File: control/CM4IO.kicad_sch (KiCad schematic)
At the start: 1 part

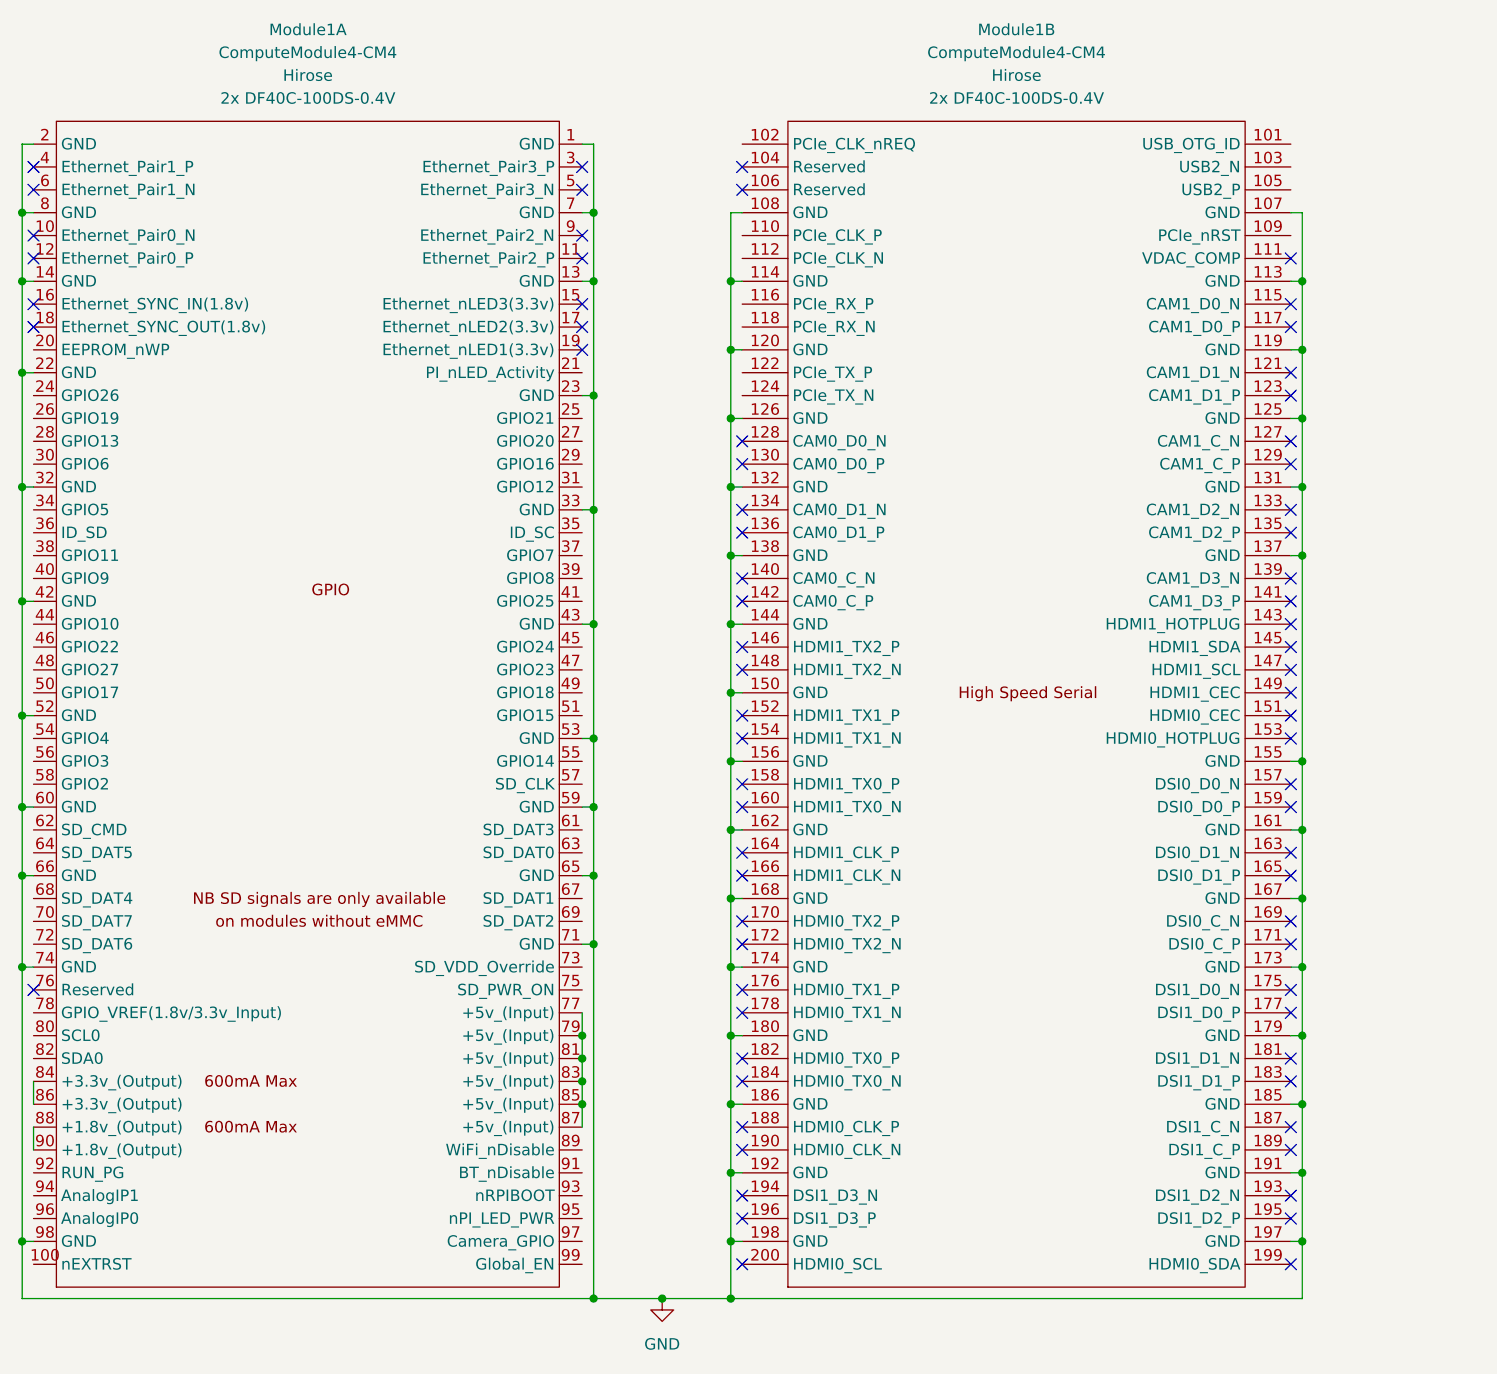
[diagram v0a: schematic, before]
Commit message: SSD
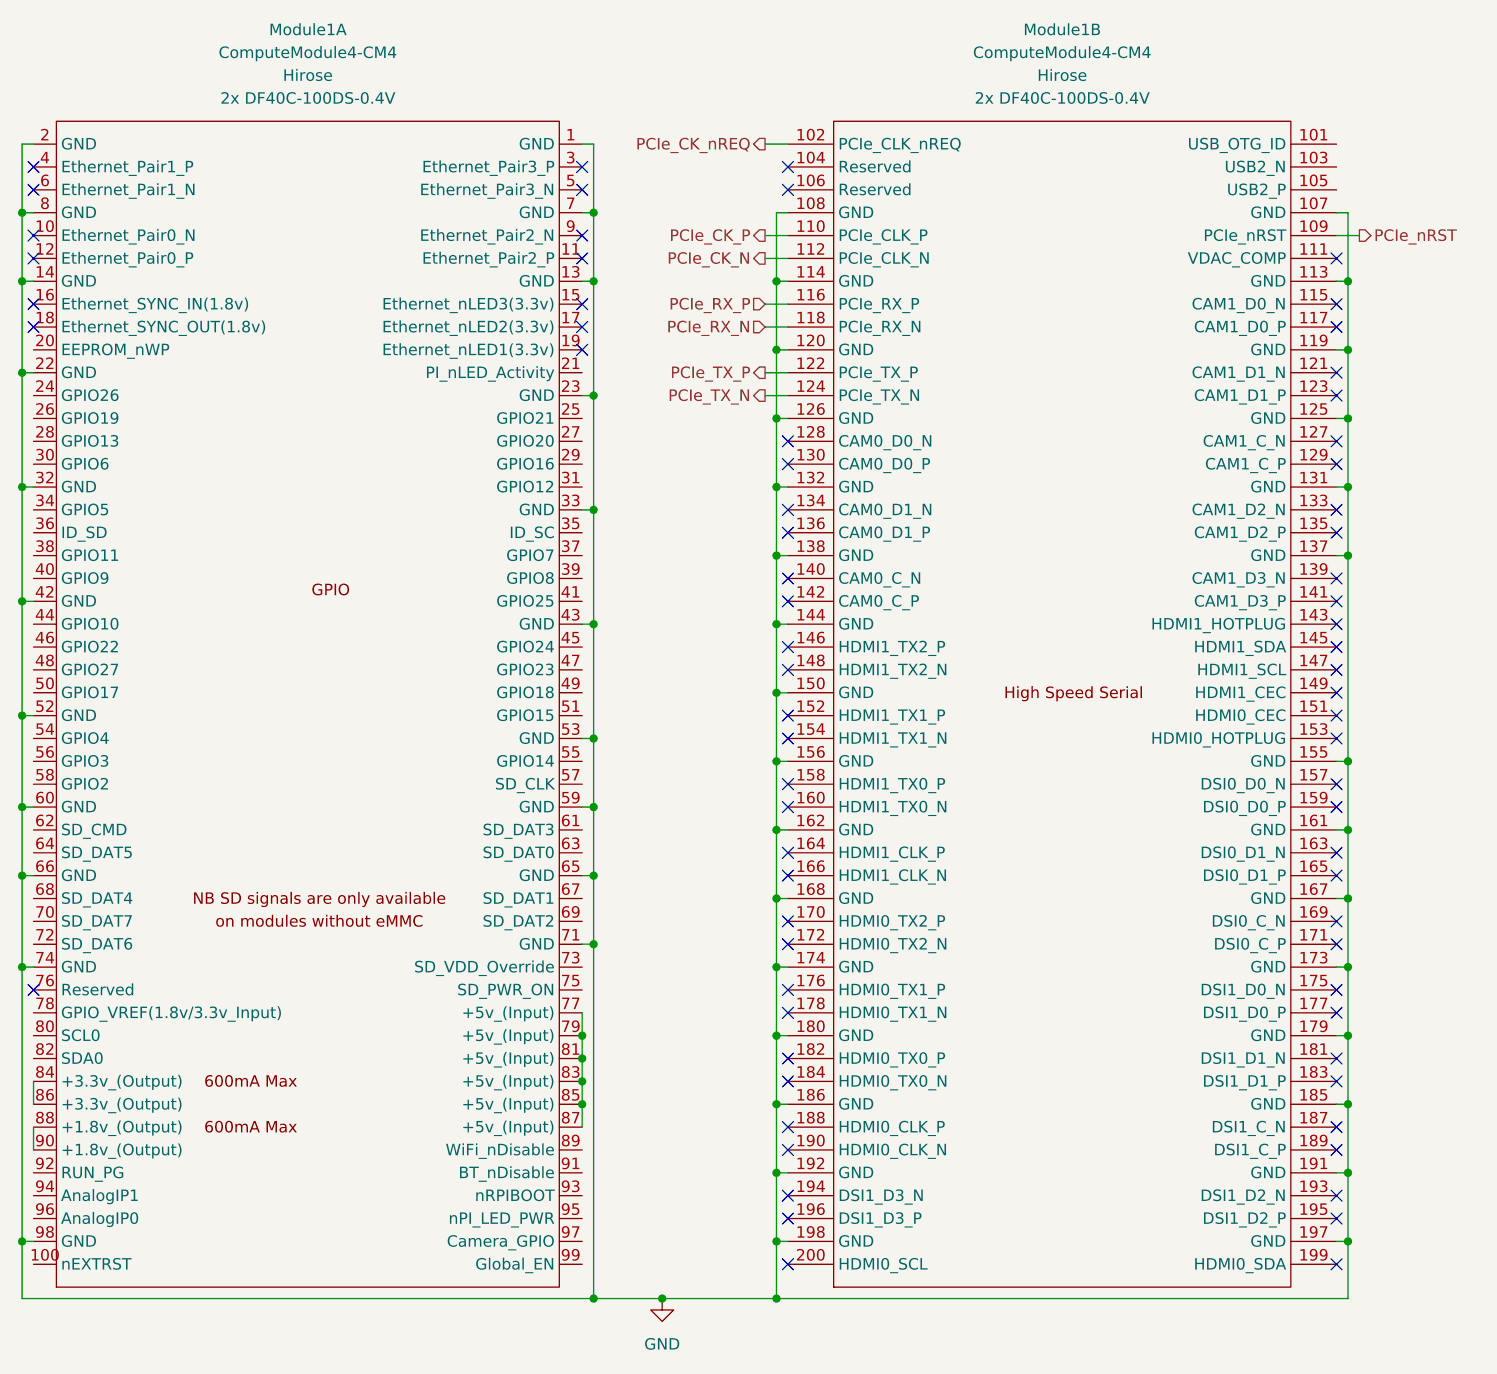
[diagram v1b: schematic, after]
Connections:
- net PCIe_CK_nREQ: now reaches Module1.102 (PCIe_CLK_nREQ)
- net PCIe_nRST: now reaches Module1.109 (PCIe_nRST)
- net PCIe_CK_P: now reaches Module1.110 (PCIe_CLK_P)
- net PCIe_CK_N: now reaches Module1.112 (PCIe_CLK_N)
- net PCIe_RX_P: now reaches Module1.116 (PCIe_RX_P)
- net PCIe_RX_N: now reaches Module1.118 (PCIe_RX_N)
- net PCIe_TX_P: now reaches Module1.122 (PCIe_TX_P)
- net PCIe_TX_N: now reaches Module1.124 (PCIe_TX_N)
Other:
- moved on the sheet: Module1B

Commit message: Component Selection
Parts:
- Module1: PN (none) -> CM4104000
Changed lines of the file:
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@@
+			)
+		)
+		(property "PN" "CM4104000"
+			(at 76.2 85.09 0)
+			(effects
+				(font
+					(size 1.27 1.27)
+				)
+				(hide yes)
 			)
 		)
@@
 			)
 		)
+		(property "PN" "CM4104000"
+			(at 17.78 90.17 0)
+			(effects
+				(font
+					(size 1.27 1.27)
+				)
+				(hide yes)
+			)
+		)
